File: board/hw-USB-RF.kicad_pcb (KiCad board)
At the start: 2 copper layers, 53 x 18 mm, 20 parts, among them J1 USB_OTG, U1 CMT2210A-ESR, U2 SPX3819, U3 ATSAMD11C14A-SS, X1 SWD, Y1 26MHz

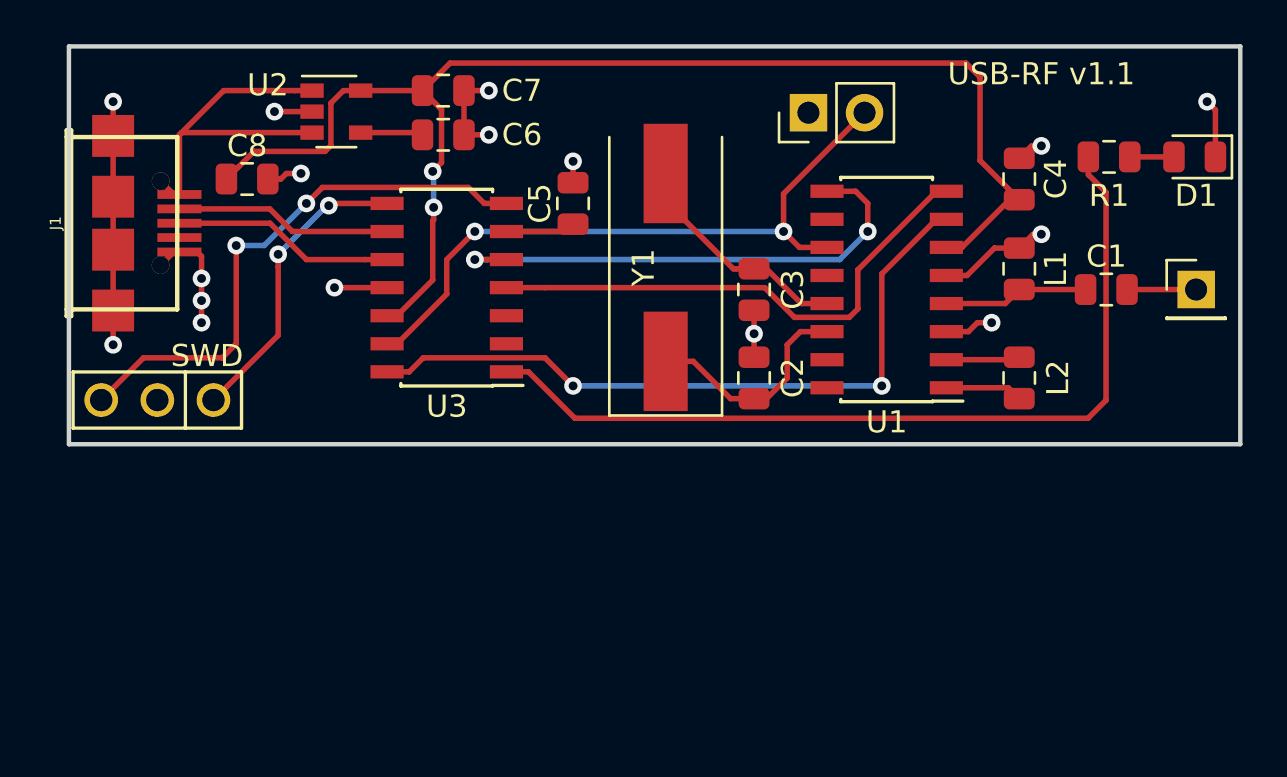
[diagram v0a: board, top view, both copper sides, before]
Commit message: WIP
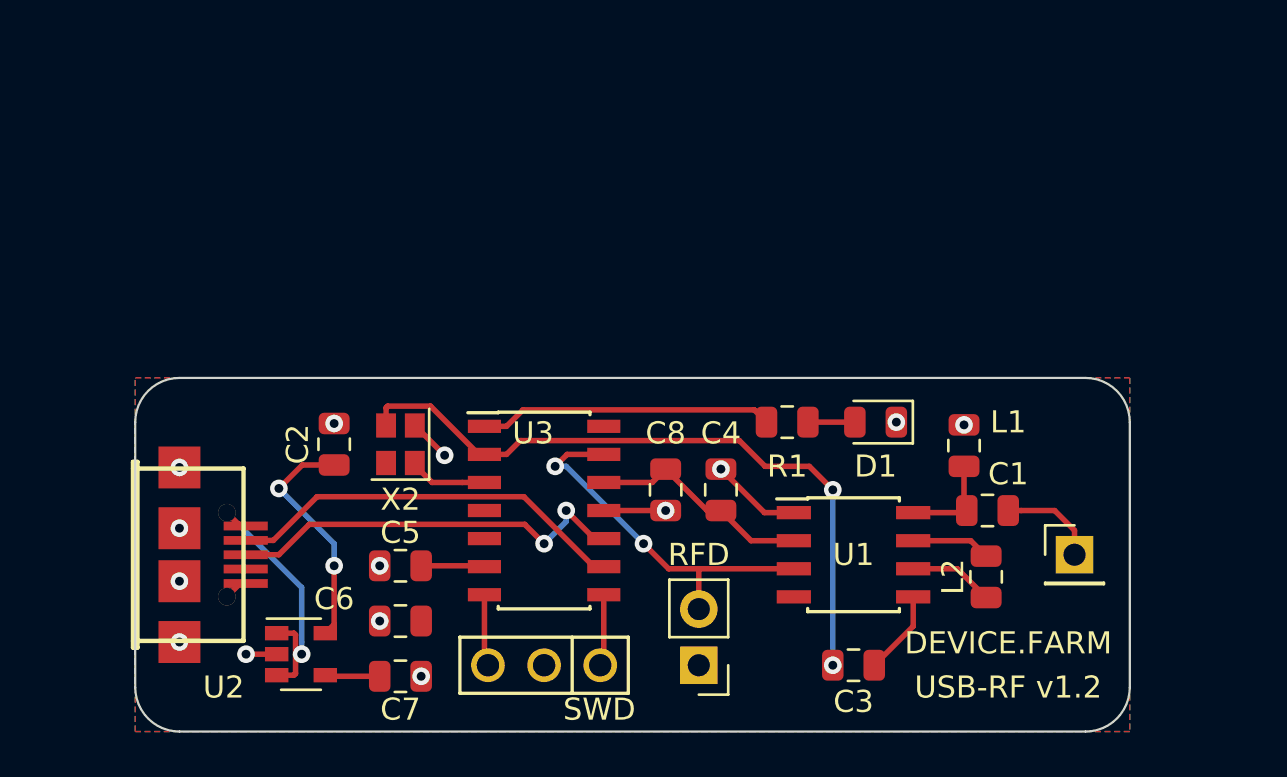
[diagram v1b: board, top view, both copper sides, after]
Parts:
- removed Y1: 26MHz, Crystal:Crystal_SMD_HC49-SD
- added X2: SG-210STF, Oscillator:Oscillator_SMD_SeikoEpson_SG210-4Pin_2.5x2.0mm, F.Cu at (123.0, 89.0)
- C2, C3: value 27p -> 100n
- U1: value CMT2210A-ESR -> CMT2210L; footprint Package_SO:SOIC-16_3.9x9.9mm_P1.27mm -> Package_SO:SOIC-8_3.9x4.9mm_P1.27mm
- moved TP1 25.5 mm to (136.5, 99.0), turned to 180 degrees
- moved U2 24.6 mm to (118.5, 98.5)
- moved C6 24.6 mm to (123.0, 99.5)
- moved C7 24.1 mm to (123.0, 97.0), turned to 180 degrees
- moved C8 23.6 mm to (135.0, 91.1), turned to 270 degrees
- moved X1 21.2 mm to (129.5, 99.0)
- moved C4 19.5 mm to (137.5, 91.1)
- moved C2 19.2 mm to (120.0, 89.0)
- moved R1 18.9 mm to (140.5, 88.0)
- moved D1 18.8 mm to (144.5, 88.0)
- moved C5 18.2 mm to (123.0, 94.5), turned to 180 degrees
- moved C3 17.6 mm to (143.5, 99.0), turned to 180 degrees
- moved J1 15.3 mm to (113.0, 94.0)
- moved AE1 13.2 mm to (153.5, 94.0)
- moved U1 12.1 mm to (143.5, 94.0), turned to 0 degrees
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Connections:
- C2 pad 1: Net-(C2-Pad1) -> +3V3
- C3 pad 2: GND -> /26MHZ
- J1 pad 4: Net-(J1-Pad4) -> (no net)
- U1 pad 1: Net-(L2-Pad1) -> GND
- U1 pad 2: Net-(L2-Pad2) -> +3V3
- U1 pad 3: GND -> /RF_DATA
- U1 pad 4: Net-(C1-Pad1) -> (no net)
- U1 pad 5: GND -> Net-(C3-Pad1)
- U1 pad 6: +3V3 -> Net-(L2-Pad2)
- U1 pad 7: /RF_CSB -> Net-(L2-Pad1)
- U1 pad 8: /RF_SDA -> Net-(C1-Pad1)
- U3 pad 14: /RF_CSB -> (no net)
- U3 pad 2: Net-(U3-Pad2) -> /26MHZ
- U3 pad 3: Net-(U3-Pad3) -> /OSC_EN
- U3 pad 4: /RF_SDA -> (no net)
- U3 pad 5: /RF_SCL -> (no net)
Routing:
- net +3V3: track 60.1 -> 20.9 mm
- net /RF_CSB: track 32.2 -> 0.00 mm, vias 2 -> 0
- net /26MHZ: track 0.00 -> 31.1 mm, vias 0 -> 2
- net GND: track 40.4 -> 11.3 mm, vias 16 -> 14
- net /LED: track 39.7 -> 13.3 mm
- net /RF_SDA: track 23.9 -> 0.00 mm
- net /RF_SCL: track 23.1 -> 0.00 mm, vias 2 -> 0
- net /SWCLK: track 25.2 -> 3.26 mm, vias 2 -> 0
- net /RF_DATA: track 30.1 -> 17.0 mm
- net /SWDIO: track 13.7 -> 3.26 mm, vias 2 -> 0
- net Net-(C2-Pad1): track 10.1 -> 0.00 mm
- net /USB_DM: track 9.82 -> 18.3 mm
- net /USB_DP: track 10.1 -> 18.6 mm, vias 0 -> 2
- net Net-(C3-Pad1): track 10.5 -> 3.83 mm
- net +5V: track 16.7 -> 12.7 mm, vias 0 -> 1
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- added copper zone on F.Cu, net +3V3
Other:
- board size 53 x 18 mm -> 45 x 16 mm
- rule pad_to_mask_clearance: 0.051 -> 0
- board text added: "DEVICE.FARM"
- board text added: "RFD"
- board text added: "USB-RF v1.2"
- board text removed: "USB-RF v1.1"
